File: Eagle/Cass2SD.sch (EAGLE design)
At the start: 34 parts, among them IC1 LM358N, Q1 8MHz, Q2 BC557C, Q3 BC447, Q4 BC447, SW1 EC12E_SW, U1 ATMEGA328P-PU, U3 MCP1702-5002, X1 MAB5SH

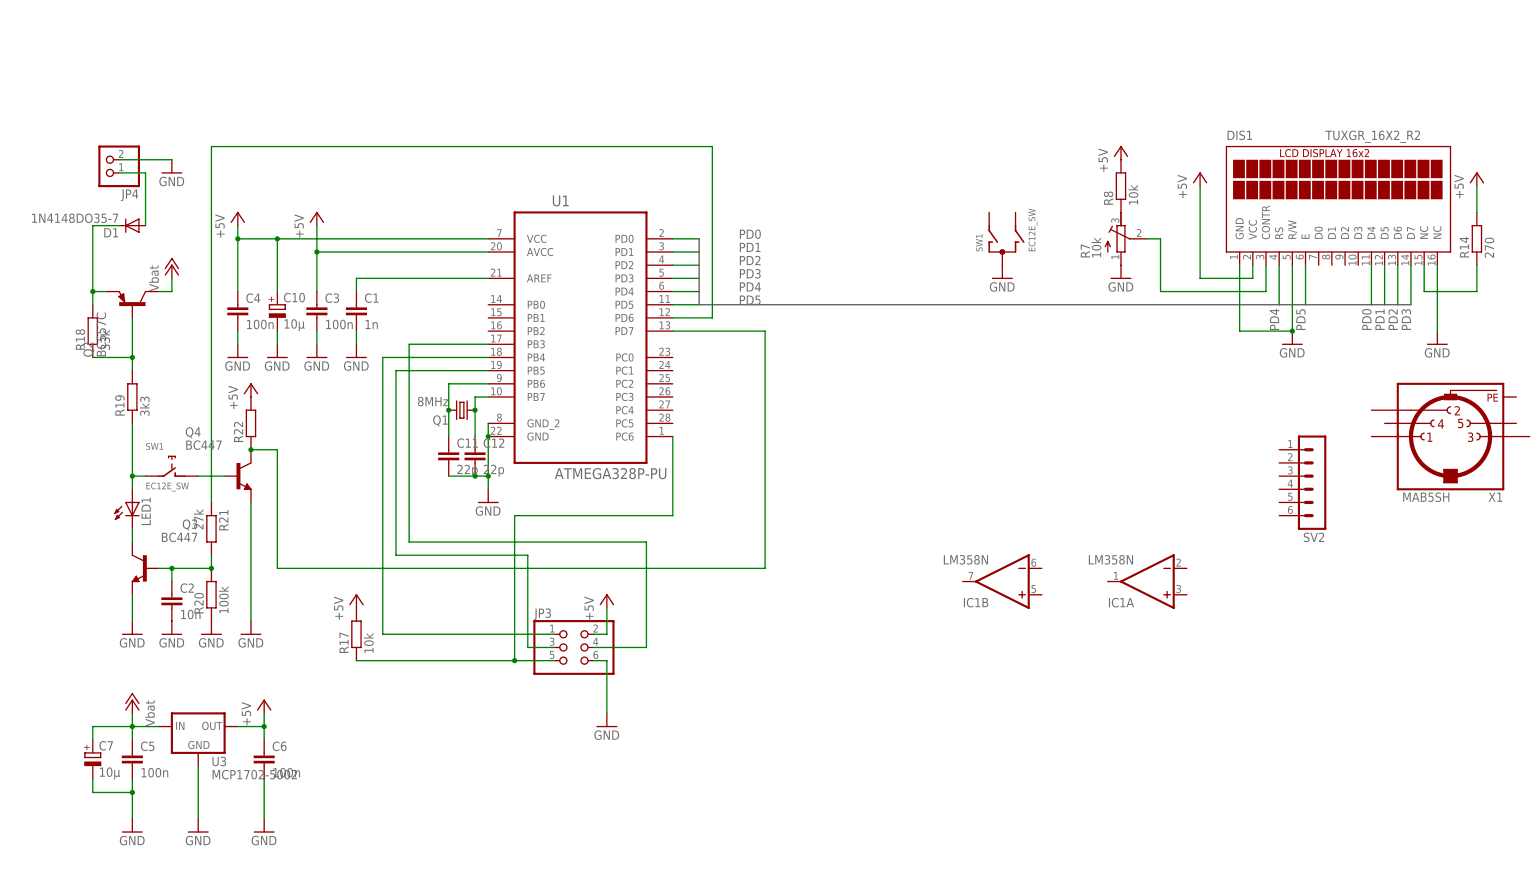
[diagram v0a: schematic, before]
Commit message: Eagle files updated/added
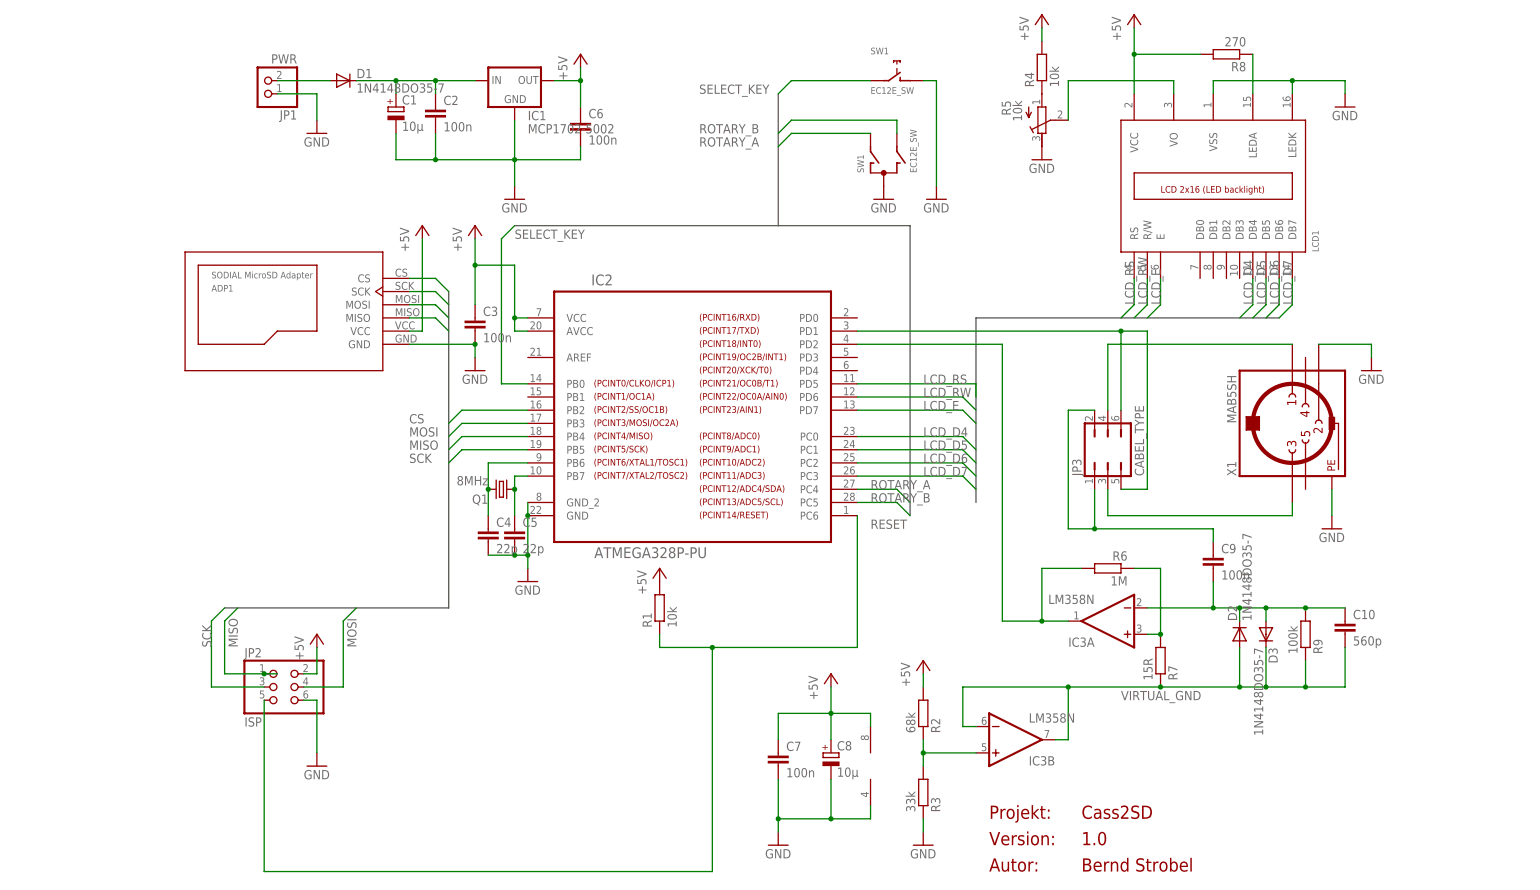
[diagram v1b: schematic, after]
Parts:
- removed C11, C12: 22p, resistor:C-EU050-025X075
- removed DIS1: TUXGR_16X2_R2, display-lcd:TUXGR_16X2_R2
- removed JP4: (no value), pinhead:PINHD-1X2
- removed LED1: (no value), led:LED5MM
- removed Q2: BC557C, transistor-pnp:BC557C
- removed Q3, Q4: BC447, transistor-npn:BC447
- removed R14: 270, resistor:R-EU_0309/12
- removed R17: 10k, resistor:R-EU_M1206
- removed R18: 33k, resistor:R-EU_M1206
- removed R19: 3k3, resistor:R-EU_M1206
- removed R20: 100k, resistor:R-EU_M1206
- removed R21: 27k, resistor:R-EU_M1206
- removed R22: (no value), resistor:R-EU_M1206
- removed SV2: (no value), con-lstb:MA06-1
- removed U1: ATMEGA328P-PU, Atmel_By_element14_Batch_1-00:ATMEGA328P-PU
- removed U3: MCP1702-5002, AdditionalSymbols:MCP1702
- added ADP1: SODIAL_MICROSD_SPI_ADAPTER, BerndAdditionalSymbols:SODIAL_MICROSD_SPI_ADAPTER
- added C8: 10µ, resistor:CPOL-EUE2.5-7
- added C9: 100n, resistor:C-EU050-025X075
- added D2, D3: 1N4148DO35-7, diode:1N4148DO35-7
- added IC2: ATMEGA328P-PU, BerndAdditionalSymbols:ATMEGA328P-PU
- added IC3: LM358N, linear:LM358N
- added JP1: PWR, pinhead:PINHD-1X2
- added JP2: ISP, pinhead:PINHD-2X3
- added LCD1: LCD_2X16, BerndAdditionalSymbols:LCD_2X16
- added R1, R4: 10k, resistor:R-EU_0207/10
- added R2: 68k, resistor:R-EU_0207/10
- added R3: 33k, resistor:R-EU_0207/10
- added R5: 10k, resistor:R-TRIMM64P
- added R6: 1M, resistor:R-EU_0207/10
- added R9: 100k, resistor:R-EU_0207/10
- C1: value 1n -> 10µ; device resistor:C-EU050-025X075 -> resistor:CPOL-EUE2.5-7
- C10: value 10µ -> 560p; device resistor:CPOL-EUE10-20 -> resistor:C-EU050-025X075
- C2: value 10n -> 100n
- C4, C5: value 100n -> 22p
- C7: value 10µ -> 100n; device resistor:CPOL-EUE10-20 -> resistor:C-EU050-025X075
- IC1: value LM358N -> MCP1702-5002; device linear:LM358N -> AdditionalSymbols:MCP1702
- JP3: value (none) -> CABEL_TYPE; device pinhead:PINHD-2X3 -> jumper:JP3Q
- R7: value 10k -> 15R; device resistor:R-TRIMM64P -> resistor:R-EU_0207/10
- R8: value 10k -> 270; device resistor:R-EU_0309/12 -> resistor:R-EU_0207/10
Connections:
- removed net +12V: C5.1, C7.+, Q2.C, U3.IN
- removed net N$15: DIS1.CONTR, R7.S
- removed net N$19: D1.A, JP4.1
- removed net N$21: D1.C, Q2.E, R18.2
- removed net N$22: JP3.5, R17.1, U1.PC6
- removed net N$23: Q2.B, R18.1, R19.2
- removed net N$24: LED1.A, R19.1, SW1G$2.2
- removed net N$25: LED1.C, Q3.C
- removed net N$26: C2.1, Q3.B, R20.2, R21.2
- removed net N$27: U1.PD6
- removed net N$28: Q4.C, R22.1, U1.PD7
- removed net N$29: Q4.B, SW1G$2.1
- removed net PD0: DIS1.D4, U1.PD0
- removed net PD1: DIS1.D5, U1.PD1
- removed net PD2: DIS1.D6, U1.PD2
- removed net PD3: DIS1.D7, U1.PD3
- removed net PD4: DIS1.RS, U1.PD4
- removed net PD5: DIS1.E, U1.PD5
- new net CS: ADP1.CS, IC2.PB2
- new net LCD_D4: IC2.PC0, LCD1.DB4
- new net LCD_D5: IC2.PC1, LCD1.DB5
- new net LCD_D6: IC2.PC2, LCD1.DB6
- new net LCD_D7: IC2.PC3, LCD1.DB7
- new net LCD_E: IC2.PD7, LCD1.E
- new net LCD_RS: IC2.PD5, LCD1.RS
- new net LCD_RW: IC2.PD6, LCD1.R/W
- new net MISO: ADP1.MISO, IC2.PB4, JP2.1
- new net MOSI: ADP1.MOSI, IC2.PB3, JP2.4
- new net N$1: C1.+, C2.1, D1.C, IC1.IN
- new net N$16: JP3.4, X1.1
- new net N$2: C10.1, C9.2, D2.C, D3.A, IC3A.-IN, R9.2
- new net N$3: IC3B.+IN, R2.1, R3.2
- new net N$7: IC3A.+IN, R6.1, R7.2
- new net N$8: IC2.PD2, IC3A.OUT, R6.2
- new net N$9: D1.A, JP1.2
- new net RESET: IC2.PC6, JP2.5, R1.1
- new net ROTARY_A: IC2.PC4, SW1G$1.A
- new net ROTARY_B: IC2.PC5, SW1G$1.B
- new net SCK: ADP1.SCK, IC2.PB5, JP2.3
- new net SELECT_KEY: IC2.PB0, SW1G$2.2
- new net VIRTUAL_GND: C10.2, D2.A, D3.C, IC3B.-IN, IC3B.OUT, R7.1, R9.1
- net +5V: now also ADP1.VCC, C7.1, C8.+, IC1.OUT, IC2.AVCC, IC2.VCC, IC3P.V+, JP2.2, LCD1.VCC, R1.2, R2.2, R4.2; no longer C10.+, C4.1, DIS1.VCC, JP3.2, R14.2, R17.2, R22.2, U1.AVCC, U1.VCC, U3.OUT
- net GND: now also ADP1.GND, C1.-, C7.2, C8.-, IC1.GND, IC2.GND, IC2.GND_2, IC3P.V-, JP1.1, JP2.6, LCD1.LEDK, LCD1.VSS, R3.1, R5.E, SW1G$2.1, X1.2, X1.PE; no longer C1.2, C10.-, C11.2, C12.2, C7.-, DIS1.GND, DIS1.NC@2, DIS1.R/W, JP3.6, JP4.2, Q3.E, Q4.E, R20.1, R7.A, U1.GND, U1.GND_2, U3.GND
- net N$10: now also IC2.PD1, JP3.5, JP3.6; no longer JP3.4, U1.PB3
- net N$11: now also LCD1.LEDA, R8.1; no longer JP3.1, U1.PB4
- net N$12: now also X1.3; no longer U1.PB5
- net N$13: now also LCD1.VO, R5.S; no longer DIS1.NC@1, R14.1
- net N$14: now also R4.1, R5.A; no longer R7.E, R8.1
- net N$4: now also C4.1, IC2.PB6; no longer C11.1, U1.PB6
- net N$5: now also C5.1, IC2.PB7; no longer C12.1, U1.PB7
- net N$6: now also C9.1, JP3.1, JP3.2; no longer C1.1, U1.AREF
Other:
- note added: "Autor:"
- note added: "Projekt:"
- note added: "Version:"
- moved on the sheet: C2, C3, C4, C5, C6, D1, Q1, R8, SW1, X1
